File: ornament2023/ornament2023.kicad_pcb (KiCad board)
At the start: 2 copper layers, 73.3 x 73.3 mm, 19 parts, among them J1 Conn_01x03, SW1 SW_Push, SW2 SW_DPDT_x2, U1 ATtiny404-SS

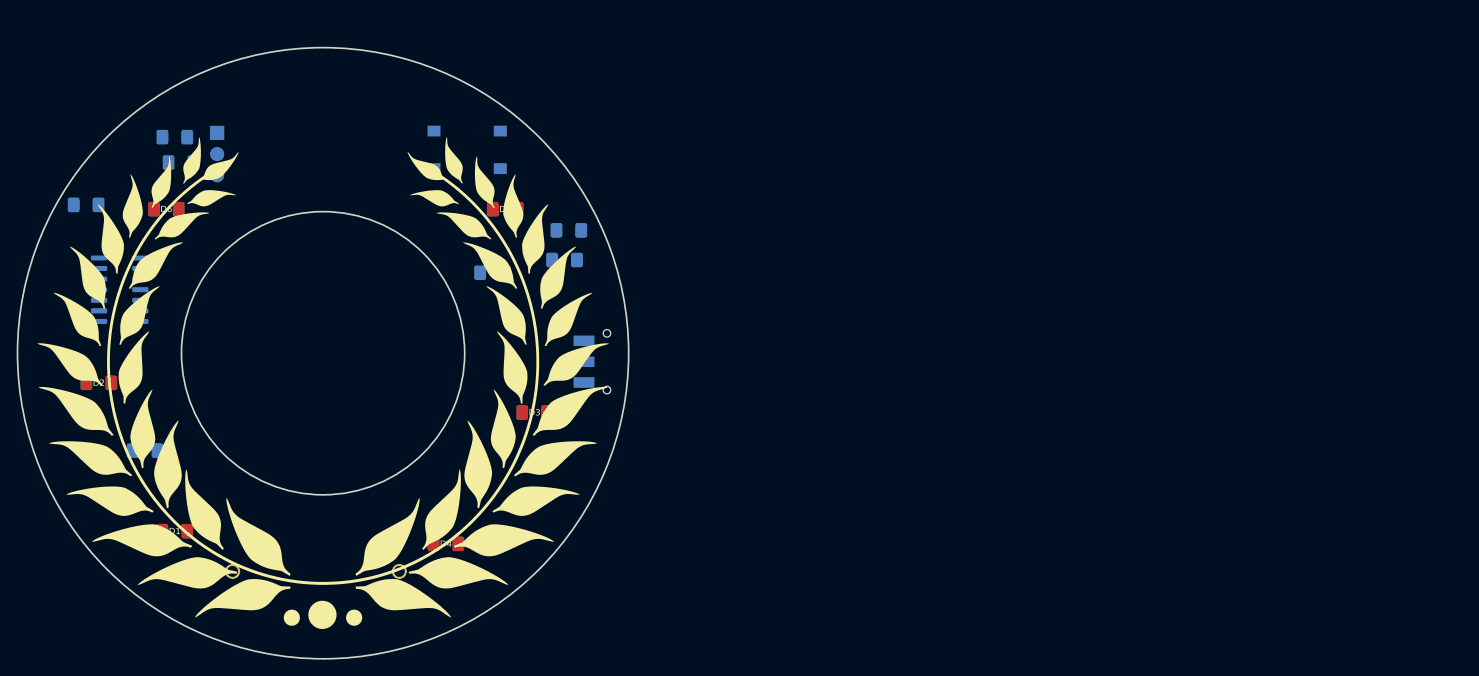
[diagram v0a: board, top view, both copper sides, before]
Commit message: kinda just sat down and did this all in one go
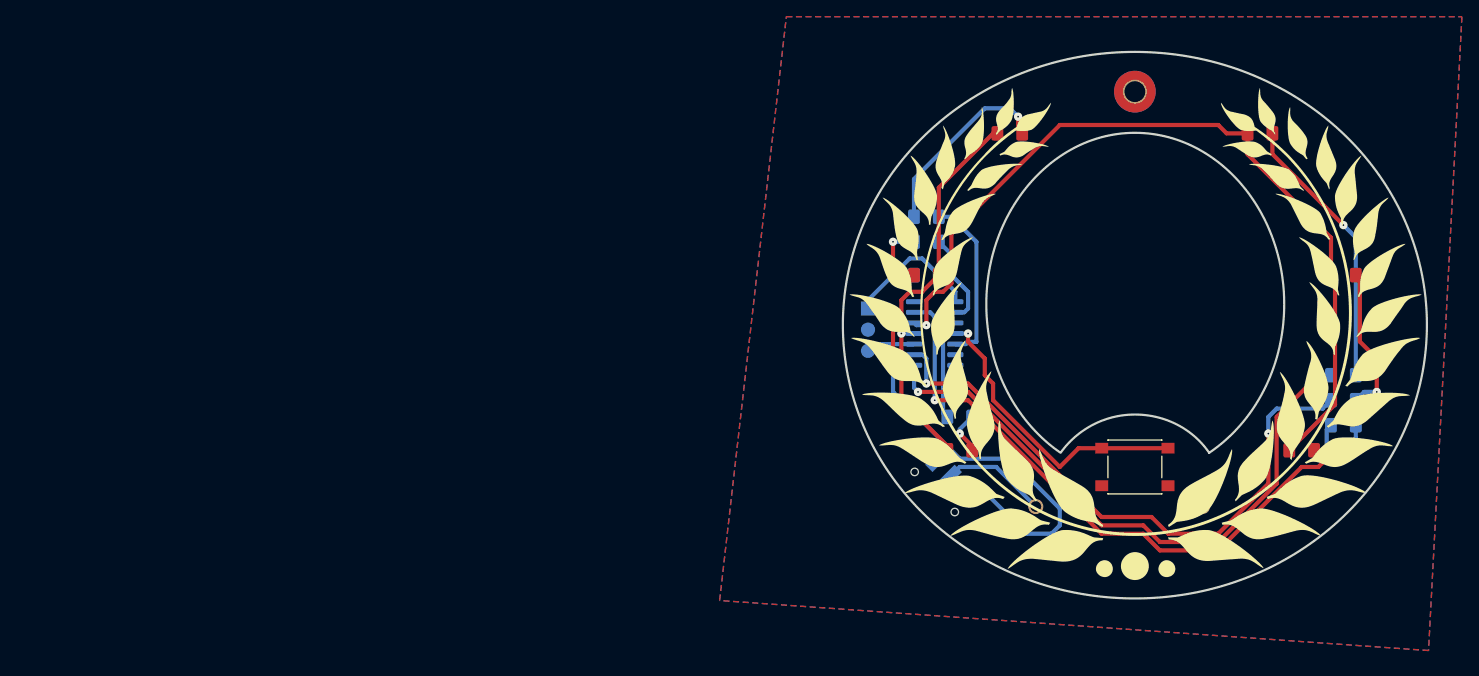
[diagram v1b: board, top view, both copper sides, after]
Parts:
- removed wreath: G***, tree:wreath
- added REF**: MountingHole_2.5mm_Pad_TopBottom, MountingHole:MountingHole_2.5mm_Pad_TopBottom, F.Cu at (203.0, 87.0)
- added svg2mod: G***, wreath:wreath, F.Cu at (203.0, 115.0)
- added svg2mod: G***, tree:Snow_flake2, B.Cu at (196.0, 88.0)
- added svg2mod: G***, tree:Snow_flake2, B.Cu at (218.0, 136.0)
- added svg2mod: G***, tree:Snow_flake2, B.Cu at (229.0, 114.0)
- added svg2mod: G***, tree:Snow_flake2, B.Cu at (183.0, 96.0)
- added svg2mod: G***, tree:Snow_flake2, B.Cu at (187.0, 131.0)
- added svg2mod: G***, tree:Snow_flake2, B.Cu at (223.0, 131.0)
- added svg2mod: G***, tree:Snow_flake2, B.Cu at (189.0, 91.0)
- added svg2mod: G***, tree:Snow_flake2, B.Cu at (209.0, 88.0)
- SW1: moved to F.Cu
- moved R5 143.8 mm to (228.0, 124.0), turned to 0 degrees
- moved R4 141.7 mm to (228.0, 121.0), turned to 0 degrees
- moved D6 139.2 mm to (223.0, 130.0)
- moved D1 110.9 mm to (188.0, 92.0)
- moved D4 109.3 mm to (218.0, 92.0)
- moved C1 101.1 mm to (178.0, 109.0)
- moved D5 100.8 mm to (228.0, 109.0)
- moved D2 100.1 mm to (178.0, 109.0), turned to 180 degrees
- moved U1 97.9 mm to (179.0, 116.0)
- moved B1 96.6 mm to (211.1, 136.8)
- moved R6 95.8 mm to (228.0, 127.0), turned to 0 degrees
- moved R2 91.0 mm to (178.0, 105.0)
- moved SW1 88.6 mm to (203.0, 132.0), turned to 0 degrees
- moved J1 80.8 mm to (171.0, 113.0)
- moved R3 58.6 mm to (182.0, 126.0), turned to 0 degrees
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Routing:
- net pin9: track 0.00 -> 100.3 mm, vias 0 -> 1
- net pin10: track 0.00 -> 75.9 mm, vias 0 -> 2
- net pin6: track 0.00 -> 73.3 mm, vias 0 -> 2
- net pin7: track 0.00 -> 71.9 mm, vias 0 -> 2
- net VCC: track 0.00 -> 70.5 mm, vias 0 -> 2
- net pin8: track 0.00 -> 47.7 mm, vias 0 -> 1
- net pin2: track 0.00 -> 36.0 mm, vias 0 -> 1
- net Net-(D4-Pad2): track 0.00 -> 33.1 mm, vias 0 -> 1
- net Net-(D1-Pad2): track 0.00 -> 23.1 mm, vias 0 -> 1
- net pin3: track 0.00 -> 20.4 mm
- net Net-(D5-Pad2): track 0.00 -> 18.0 mm, vias 0 -> 1
- net pin1: track 0.00 -> 12.6 mm
- net Net-(SW2-Pad2): track 0.00 -> 12.6 mm
- net pin0: track 0.00 -> 11.2 mm
- net Net-(D2-Pad2): track 0.00 -> 8.44 mm, vias 0 -> 1
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- added copper zone on B.Cu, net GND
- added copper zone on F.Cu, net GND
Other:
- board size 73.3 x 73.3 mm -> 70 x 65.5 mm
- board text added: "-"
- board text added: "3v3"
- board text added: "GND"
- board text added: "Hack me!"
- board text added: "JLCJLCJLCJLC"
- board text added: "Merry Christmas! Chris Johnston 2023"
- board text added: "Power"
- board text added: "UPDI"
